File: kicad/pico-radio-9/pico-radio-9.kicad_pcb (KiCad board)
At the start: 2 copper layers, 87.2 x 67 mm, 56 parts, among them J1 FM antenna, J2 SW antenna, J3 MW/SW antenna, J4 HF Amplifier, J5 Batterry, Q1 PN2222A, Q2 PN2222A, Q3 PN2222A, SW1 Reset, U1 SI4732-A10-GS, U2 TFT_320x240, U3 MCP6004, U4 KY-040, Y1 32.762kHz

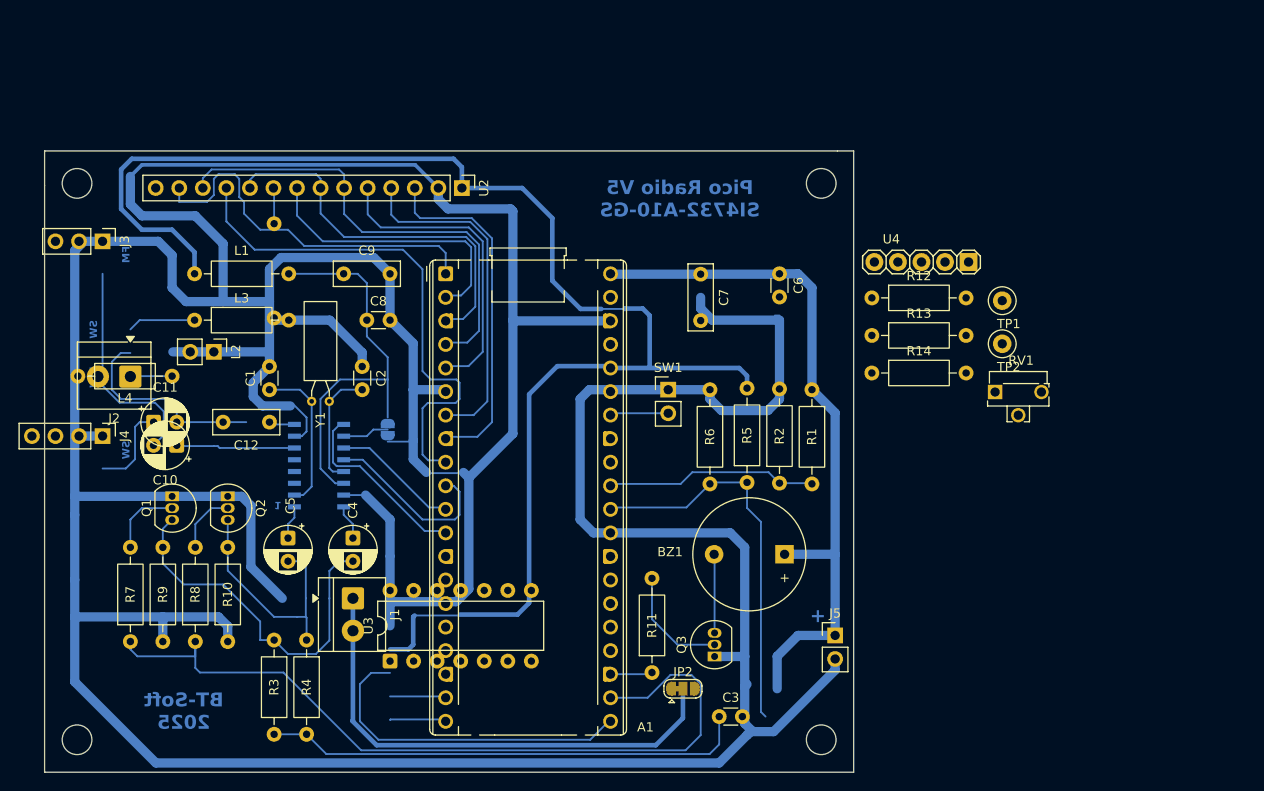
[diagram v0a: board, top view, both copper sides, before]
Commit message: Refactor code structure for improved readability and maintainability
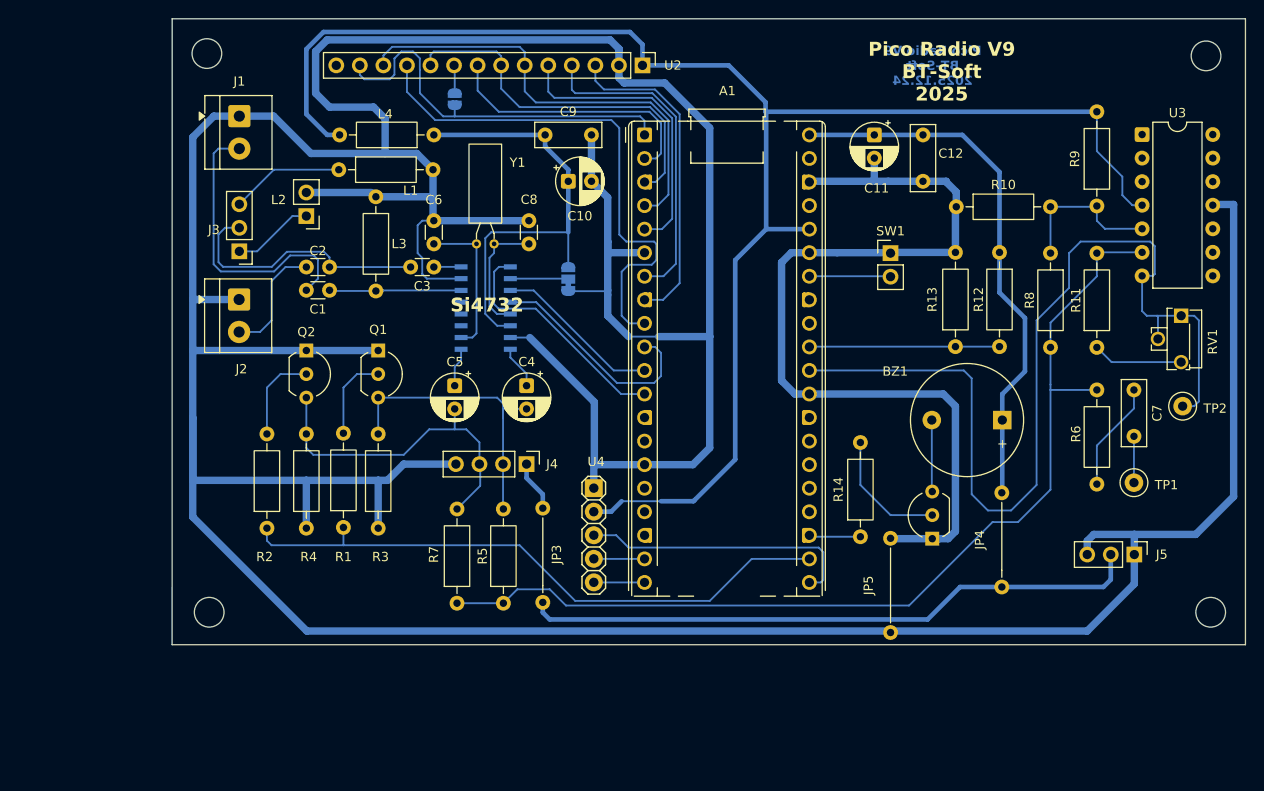
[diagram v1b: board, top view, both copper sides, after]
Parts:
- removed the REF** at (32.2, 43.8)
- removed the REF** at (112.5, 43.8)
- removed the REF** at (32.2, 103.8)
- removed the REF** at (112.5, 103.8)
- added JP4: NYÁK átkötés, Resistor_THT:R_Axial_DIN0207_L6.3mm_D2.5mm_P10.16mm_Horizontal, F.Cu at (132.0, 87.3)
- added JP5: NYÁK átkötés, Resistor_THT:R_Axial_DIN0207_L6.3mm_D2.5mm_P10.16mm_Horizontal, F.Cu at (120.0, 92.2)
- added REF**: MountingHole_3.2mm_M3, MountingHole:MountingHole_3.2mm_M3, F.Cu at (46.2, 29.8)
- added REF**: MountingHole_3.2mm_M3, MountingHole:MountingHole_3.2mm_M3, F.Cu at (154.0, 30.0)
- added REF**: MountingHole_3.2mm_M3, MountingHole:MountingHole_3.2mm_M3, F.Cu at (154.5, 90.0)
- added REF**: MountingHole_3.2mm_M3, MountingHole:MountingHole_3.2mm_M3, F.Cu at (46.5, 90.0)
- J5: footprint Connector_PinHeader_2.54mm:PinHeader_1x02_P2.54mm_Vertical -> Connector_PinHeader_2.54mm:PinHeader_1x03_P2.54mm_Vertical
- JP2: moved to B.Cu
- JP3: moved to F.Cu
- Q1, Q2, Q3: footprint Package_TO_SOT_THT:TO-92_Inline -> Package_TO_SOT_THT:TO-92_Inline_Wide
- moved R9 111.1 mm to (142.2, 46.2)
- moved R8 101.3 mm to (137.2, 51.3), turned to -90 degrees
- moved U3 99.0 mm to (147.1, 38.5), turned to 0 degrees
- moved R10 91.5 mm to (127.1, 46.3), turned to 0 degrees
- moved C11 83.7 mm to (118.2, 38.5), turned to -90 degrees
- moved C12 77.0 mm to (123.5, 38.5), turned to -90 degrees
- moved R11 59.4 mm to (142.2, 61.4)
- moved C3 57.4 mm to (70.7, 52.8), turned to 180 degrees
- moved R2 55.5 mm to (52.7, 80.9)
- moved J1 53.4 mm to (49.8, 36.5)
- moved R1 52.7 mm to (61.0, 80.9), turned to 90 degrees
- moved C10 50.9 mm to (85.2, 43.5), turned to 0 degrees
- moved C7 48.4 mm to (146.2, 66.0)
- moved U4 46.2 mm to (88.0, 80.4), turned to 90 degrees
- moved JP2 45.9 mm to (85.2, 54.1), turned to 90 degrees
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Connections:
- J5 pad 1: +Vbus -> GND
- J5 pad 2: GND -> Net-(J5-Pin_2)
- JP3 pad 2: +Vbus -> Net-(J5-Pin_2)
- R10 pad 2: Net-(U3A-+) -> Net-(U3B-+)
- R11 pad 2: Net-(U3A--) -> Net-(U3B--)
- R5 pad 1: Net-(U3A--) -> Net-(U3B--)
- R6 pad 1: Net-(U3A--) -> Net-(U3B--)
- R7 pad 1: Net-(U3A--) -> Net-(U3B--)
- R8 pad 1: Net-(U3A-+) -> Net-(U3B-+)
- R8 pad 2: Net-(U3A--) -> Net-(U3B--)
- R9 pad 1: Net-(U3A-+) -> Net-(U3B-+)
- U3 pad 1: AD_FFT_AUDIO -> (no net)
- U3 pad 2: Net-(U3A--) -> (no net)
- U3 pad 3: Net-(U3A-+) -> (no net)
- U3 pad 5: (no net) -> Net-(U3B-+)
- U3 pad 6: (no net) -> Net-(U3B--)
- U3 pad 7: (no net) -> AD_FFT_AUDIO
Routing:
- net Net-(U3B--): track 0.00 -> 108.1 mm
- net Net-(J5-Pin_2): track 0.00 -> 67.1 mm
- net AD_FFT_AUDIO: track 42.4 -> 103.7 mm
- net Net-(J1-Pin_1): track 54.3 -> 0.00 mm
- net Net-(C3-Pad1): track 52.3 -> 0.00 mm
- net Net-(JP2-B): track 0.00 -> 47.9 mm
- net Net-(JP1-B): track 43.0 -> 0.00 mm
- net GND: track 590.5 -> 625.6 mm
- net Net-(J1-Pin_2): track 0.00 -> 31.6 mm
- net +Vbus: track 86.7 -> 58.5 mm
- net AUDIO_MUTE: track 88.1 -> 66.3 mm
- net +3.3V: track 159.5 -> 176.9 mm
- net Net-(U3B-+): track 0.00 -> 17.1 mm
- net Net-(J3-Pin_3): track 0.00 -> 13.0 mm
- net Net-(J2-Pin_2): track 0.00 -> 12.6 mm
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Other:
- board size 87.2 x 67 mm -> 115.8 x 67.5 mm
- board text added: "Pico Radio V9 BT-Soft 2025"
- board text added: "Pico Radio V9 BT-Soft 2025.12.24"
- board text added: "Si4732"
- board text removed: "+"
- board text removed: "1"
- board text removed: "BT-Soft 2025"
- board text removed: "FM"
- board text removed: "MW"
- board text removed: "Pico Radio V5 SI4732-A10-GS"
- board text removed: "SW"

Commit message: Kicad PCB design
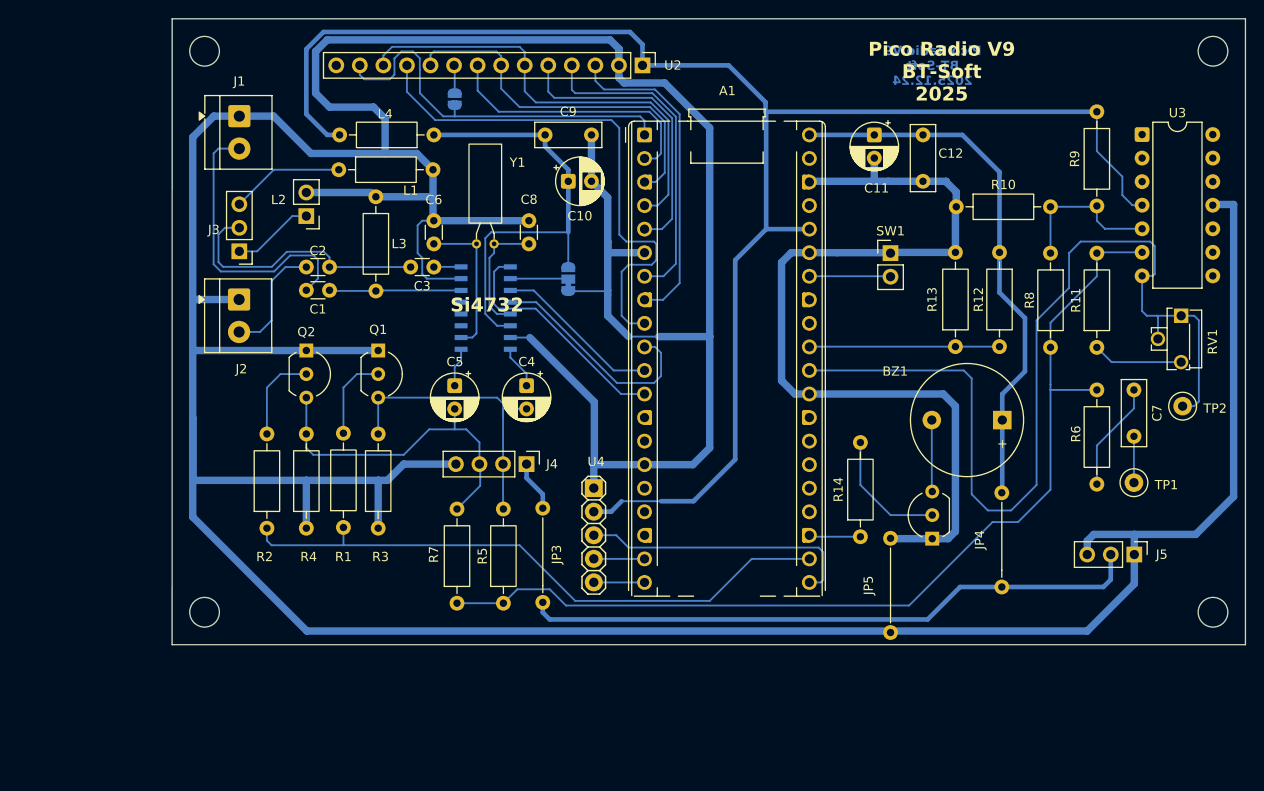
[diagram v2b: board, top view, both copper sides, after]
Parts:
- removed REF** (x4): MountingHole_3.2mm_M3, MountingHole:MountingHole_3.2mm_M3
- added H1: MountingHole, MountingHole:MountingHole_3.2mm_M3, F.Cu at (46.0, 90.0)
- added H2: MountingHole, MountingHole:MountingHole_3.2mm_M3, F.Cu at (154.8, 90.0)
- added H3: MountingHole, MountingHole:MountingHole_3.2mm_M3, F.Cu at (46.0, 29.5)
- added H4: MountingHole, MountingHole:MountingHole_3.2mm_M3, F.Cu at (154.8, 29.5)
- J3: value MW/SW antenna -> MW/SW antenna kapcsoló
- L2: value 30uH (MW Ferrite antenna) -> 30uH (MW Ferrit antenna)
